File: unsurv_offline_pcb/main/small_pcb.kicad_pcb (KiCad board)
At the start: 4 copper layers, 35 x 45 mm, 51 parts, among them J1 USB_B_Micro, Q1 Q_PMOS_GSD, Q2 UMH3N, SW1 SW_DIP_x01, U1 MCP73831-2-OT, U2 AP2112K-3.3, U3 MPU-6050_NRND, U4 ESP32-WROOM-32, U5 RF430CL330H, U6 CAM-M8C-0-10, U7 CH340G

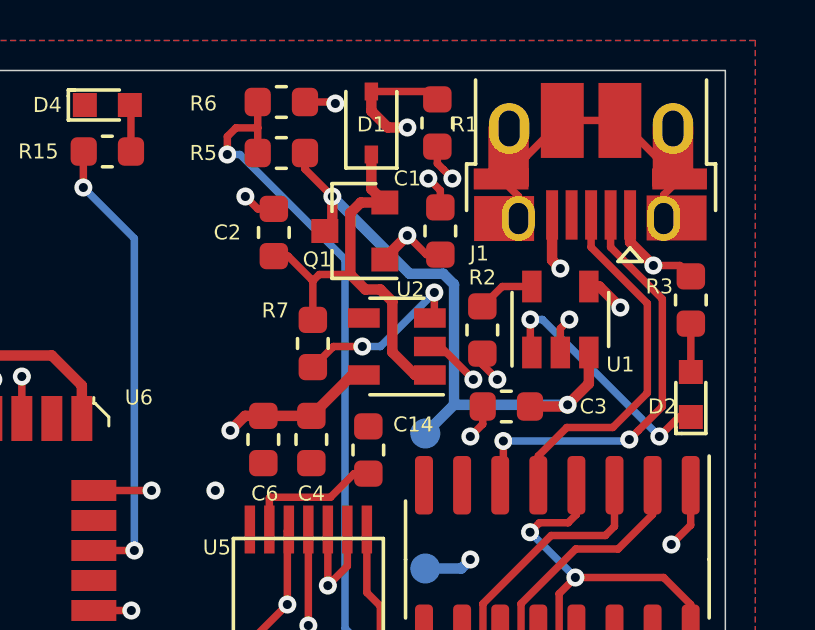
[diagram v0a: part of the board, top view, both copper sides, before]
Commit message: updated 3D files + exported schematic
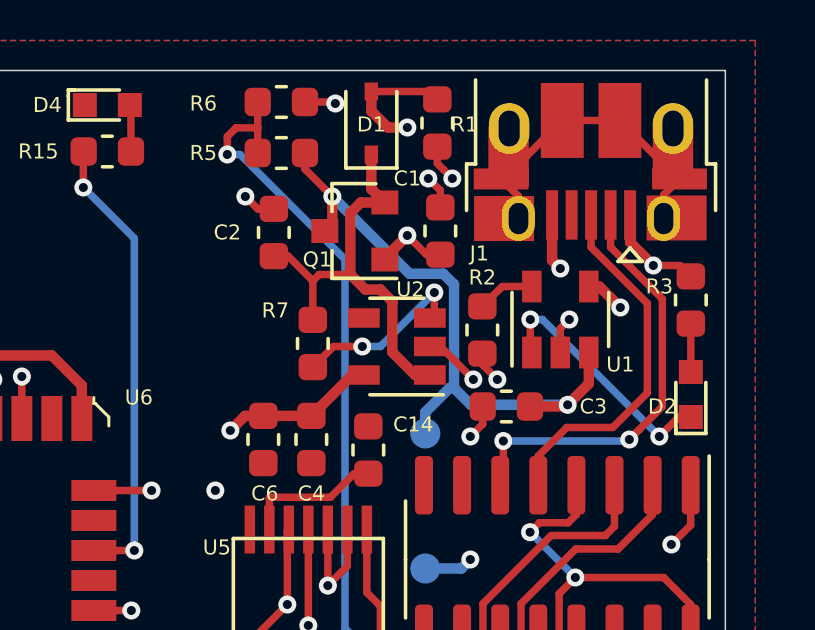
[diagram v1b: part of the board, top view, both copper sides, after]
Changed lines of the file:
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@@
     (thickness 1.6)
     (drawings 12)
-    (tracks 613)
+    (tracks 616)
     (zones 0)
     (modules 51)
@@
   )
   (setup
-    (last_trace_width 0.25)
+    (last_trace_width 0.35)
     (user_trace_width 0.35)
     (user_trace_width 0.5)
@@
   (segment (start 79.74375 61.14375) (end 79.6875 61.2) (width 0.35) (layer F.Cu) (net 3))
   (via (at 79.74375 61.14375) (size 0.6) (drill 0.3) (layers F.Cu B.Cu) (net 3))
-  (segment (start 75.95625 61.14375) (end 79.74375 61.14375) (width 0.35) (layer B.Cu) (net 3))
-  (segment (start 75 62.1) (end 75.95625 61.14375) (width 0.35) (layer B.Cu) (net 3))
   (via (at 71.9 54.2) (size 0.6) (drill 0.3) (layers F.Cu B.Cu) (net 3))
-  (segment (start 75.600001 56.774999) (end 74.474999 56.774999) (width 0.35) (layer B.Cu) (net 3))
-  (segment (start 75.95625 61.14375) (end 75.95625 57.131248) (width 0.35) (layer B.Cu) (net 3))
-  (segment (start 74.474999 56.774999) (end 71.9 54.2) (width 0.35) (layer B.Cu) (net 3))
-  (segment (start 75.95625 57.131248) (end 75.600001 56.774999) (width 0.35) (layer B.Cu) (net 3))
   (segment (start 71.9 55.1) (end 71.65 55.35) (width 0.35) (layer F.Cu) (net 3))
   (segment (start 71.9 54.2) (end 71.9 55.1) (width 0.35) (layer F.Cu) (net 3))
   (segment (start 70.9875 53.2875) (end 71.9 54.2) (width 0.25) (layer F.Cu) (net 3))
   (segment (start 70.9875 52.75) (end 70.9875 53.2875) (width 0.25) (layer F.Cu) (net 3))
+  (segment (start 76.518748 61.14375) (end 79.74375 61.14375) (width 0.35) (layer B.Cu) (net 3))
+  (segment (start 74.474999 56.774999) (end 75.600001 56.774999) (width 0.35) (layer B.Cu) (net 3))
+  (segment (start 71.9 54.2) (end 74.474999 56.774999) (width 0.35) (layer B.Cu) (net 3))
+  (segment (start 75.600001 56.774999) (end 75.95625 57.131248) (width 0.35) (layer B.Cu) (net 3))
+  (segment (start 75.95625 57.131248) (end 75.95625 60.581252) (width 0.35) (layer B.Cu) (net 3))
+  (segment (start 75.95625 60.581252) (end 76.518748 61.14375) (width 0.35) (layer B.Cu) (net 3))
+  (segment (start 75.811642 60.581252) (end 75.95625 60.581252) (width 0.35) (layer B.Cu) (net 3))
+  (segment (start 75 61.392894) (end 75.811642 60.581252) (width 0.35) (layer B.Cu) (net 3))
+  (segment (start 75 62.1) (end 75 61.392894) (width 0.35) (layer B.Cu) (net 3))
   (segment (start 69.0875 81.525) (end 69.0875 81.05) (width 0.25) (layer F.Cu) (net 4))
   (segment (start 69.3125 81.75) (end 69.0875 81.525) (width 0.25) (layer F.Cu) (net 4))
